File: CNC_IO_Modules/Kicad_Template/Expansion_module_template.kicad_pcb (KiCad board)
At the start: 2 copper layers, 32 x 42 mm, 2 parts

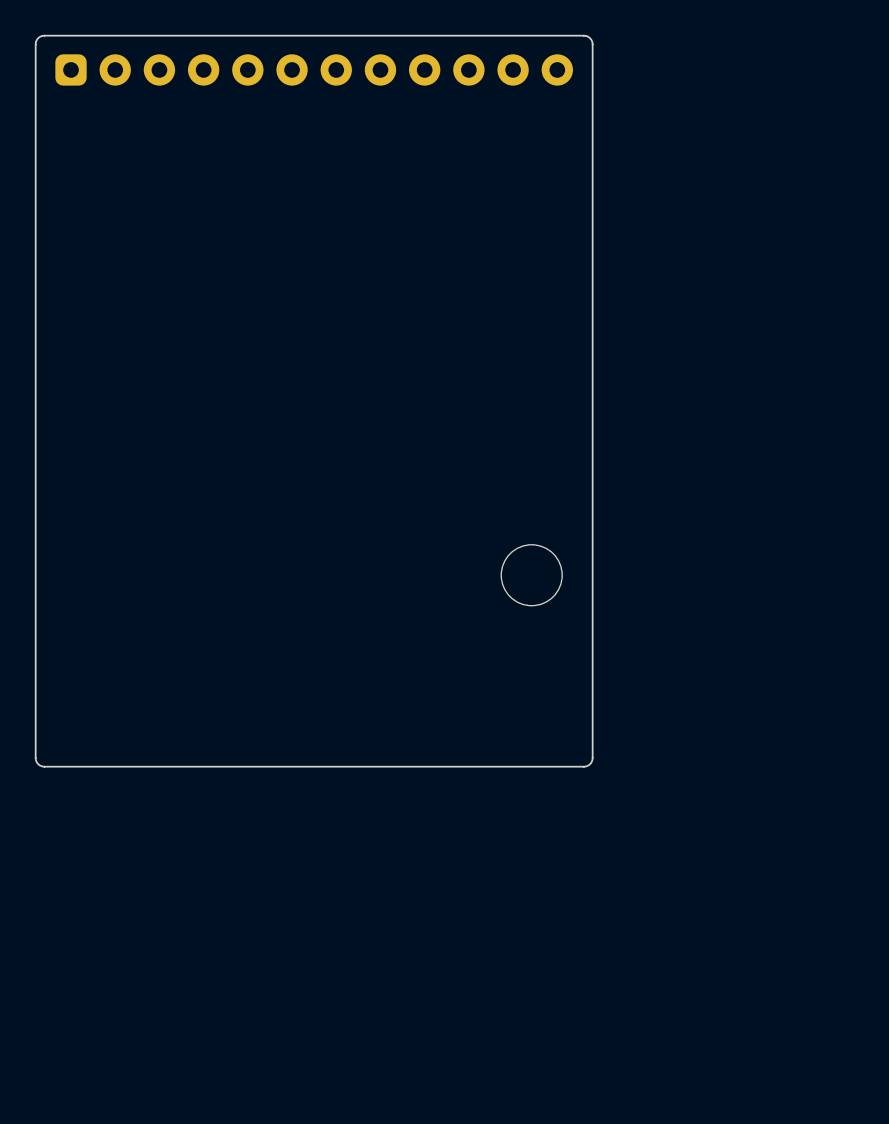
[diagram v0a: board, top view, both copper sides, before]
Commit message: Add Kicad versions
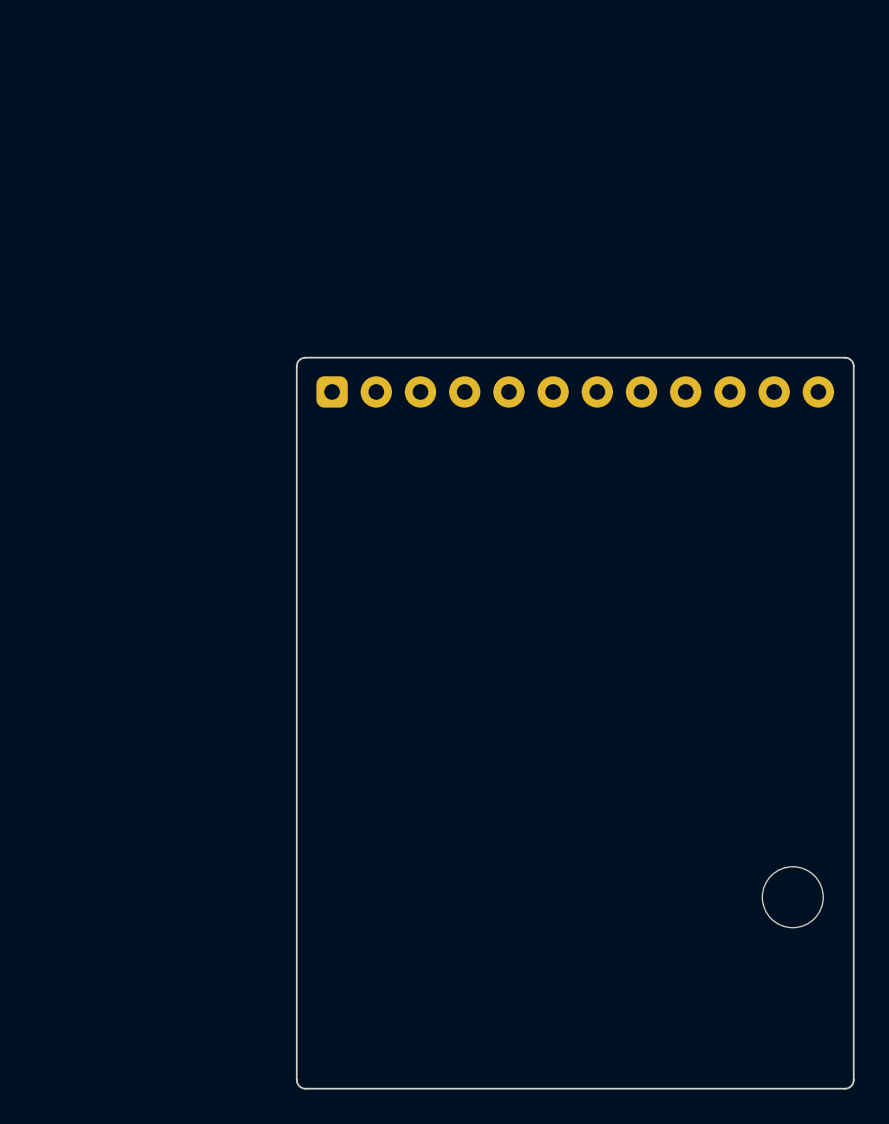
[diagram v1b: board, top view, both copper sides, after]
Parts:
- moved REF** 23.8 mm to (143.5, 107.5)
- moved REF** 23.8 mm to (117.0, 78.5)
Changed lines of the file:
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@@
   (net 0 "")
   (footprint "MountingHole:MountingHole_3.5mm" (layer "F.Cu")
-    (at 128.5 89)
+    (at 143.5 107.5)
     (descr "Mounting Hole 3.5mm, no annular")
     (tags "mounting hole 3.5mm no annular")
@@
   )
   (footprint "Connector_PinHeader_2.54mm:PinHeader_1x12_P2.54mm_Vertical" (layer "F.Cu")
-    (at 102.02998 59.97001 90)
+    (at 117.02998 78.47001 90)
     (descr "Through hole straight pin header, 1x12, 2.54mm pitch, single row")
     (tags "Through hole pin header THT 1x12 2.54mm single row")
@@
     )
   )
-  (gr_circle (center 128.49999 88.99999) (end 130.24998 88.99999) (layer "B.Mask") (width 0) (fill solid))
-  (gr_circle (center 128.49999 88.99999) (end 130.24998 88.99999) (layer "F.Mask") (width 0) (fill solid))
-  (gr_arc (start 100.5 100) (mid 100.146447 99.853553) (end 100 99.5) (layer "Edge.Cuts") (width 0.1))
-  (gr_arc (start 132 99.5) (mid 131.853553 99.853553) (end 131.5 100) (layer "Edge.Cuts") (width 0.1))
-  (gr_line (start 132 58.5) (end 132 99.5) (layer "Edge.Cuts") (width 0.1))
-  (gr_line (start 100.5 58) (end 131.5 58) (layer "Edge.Cuts") (width 0.1))
-  (gr_line (start 131.5 100) (end 100.5 100) (layer "Edge.Cuts") (width 0.1))
-  (gr_arc (start 100 58.5) (mid 100.146447 58.146447) (end 100.5 58) (layer "Edge.Cuts") (width 0.1))
-  (gr_arc (start 131.5 58) (mid 131.853553 58.146447) (end 132 58.5) (layer "Edge.Cuts") (width 0.1))
-  (gr_line (start 100 99.5) (end 100 58.5) (layer "Edge.Cuts") (width 0.1))
-  (gr_text "5" (at 119.729 56.391272) (layer "Dwgs.User")
+  (gr_circle (center 143.49999 107.49999) (end 145.24998 107.49999) (layer "B.Mask") (width 0) (fill solid))
+  (gr_circle (center 143.49999 107.49999) (end 145.24998 107.49999) (layer "F.Mask") (width 0) (fill solid))
+  (gr_arc (start 115.5 118.5) (mid 115.146447 118.353553) (end 115 118) (layer "Edge.Cuts") (width 0.1))
+  (gr_arc (start 147 118) (mid 146.853553 118.353553) (end 146.5 118.5) (layer "Edge.Cuts") (width 0.1))
+  (gr_line (start 147 77) (end 147 118) (layer "Edge.Cuts") (width 0.1))
+  (gr_line (start 115.5 76.5) (end 146.5 76.5) (layer "Edge.Cuts") (width 0.1))
+  (gr_line (start 146.5 118.5) (end 115.5 118.5) (layer "Edge.Cuts") (width 0.1))
+  (gr_arc (start 115 77) (mid 115.146447 76.646447) (end 115.5 76.5) (layer "Edge.Cuts") (width 0.1))
+  (gr_arc (start 146.5 76.5) (mid 146.853553 76.646447) (end 147 77) (layer "Edge.Cuts") (width 0.1))
+  (gr_line (start 115 118) (end 115 77) (layer "Edge.Cuts") (width 0.1))
+  (gr_text "5" (at 134.729 74.891272) (layer "Dwgs.User")
     (effects (font (size 1 1) (thickness 0.15)))
   )
-  (gr_text "3" (at 114.522 56.391272) (layer "Dwgs.User")
+  (gr_text "3" (at 129.522 74.891272) (layer "Dwgs.User")
     (effects (font (size 1 1) (thickness 0.15)))
   )
-  (gr_text "VMOT" (at 104.616 55.32901 90) (layer "Dwgs.User")
+  (gr_text "VMOT" (at 119.616 73.82901 90) (layer "Dwgs.User")
     (effects (font (size 1 1) (thickness 0.15)))
   )
-  (gr_text "GND" (at 130.016 55.709963 90) (layer "Dwgs.User")
+  (gr_text "GND" (at 145.016 74.209963 90) (layer "Dwgs.User")
     (effects (font (size 1 1) (thickness 0.15)))
   )
-  (gr_text "7" (at 124.809 56.391272) (layer "Dwgs.User")
+  (gr_text "7" (at 139.809 74.891272) (layer "Dwgs.User")
     (effects (font (size 1 1) (thickness 0.15)))
   )
-  (gr_text "8" (at 127.476 56.391272) (layer "Dwgs.User")
+  (gr_text "8" (at 142.476 74.891272) (layer "Dwgs.User")
     (effects (font (size 1 1) (thickness 0.15)))
   )
-  (gr_text "5V" (at 107.156 56.32901 90) (layer "Dwgs.User")
+  (gr_text "5V" (at 122.156 74.82901 90) (layer "Dwgs.User")
     (effects (font (size 1 1) (thickness 0.15)))
   )
-  (gr_text "6" (at 122.396 56.391272) (layer "Dwgs.User")
+  (gr_text "6" (at 137.396 74.891272) (layer "Dwgs.User")
     (effects (font (size 1 1) (thickness 0.15)))
   )
-  (gr_text "2" (at 112.109 56.391272) (layer "Dwgs.User")
+  (gr_text "2" (at 127.109 74.891272) (layer "Dwgs.User")
     (effects (font (size 1 1) (thickness 0.15)))
   )
-  (gr_text "1" (at 109.569 56.391272) (layer "Dwgs.User")
+  (gr_text "1" (at 124.569 74.891272) (layer "Dwgs.User")
     (effects (font (size 1 1) (thickness 0.15)))
   )
-  (gr_text "4" (at 117.189 56.391272) (layer "Dwgs.User")
+  (gr_text "4" (at 132.189 74.891272) (layer "Dwgs.User")
     (effects (font (size 1 1) (thickness 0.15)))
   )
-  (gr_text "GND" (at 102.076 55.709963 90) (layer "Dwgs.User")
+  (gr_text "GND" (at 117.076 74.209963 90) (layer "Dwgs.User")
     (effects (font (size 1 1) (thickness 0.15)))
   )
+  (dimension (type aligned) (layer "Dwgs.User")
+    (pts (xy 115 118) (xy 147 118))
+    (height 5.12)
+    (gr_text "32,0000 mm" (at 131 121.97) (layer "Dwgs.User")
+      (effects (font (size 1 1) (thickness 0.15)))
+    )
+    (format (units 3) (units_format 1) (precision 4))
+    (style (thickness 0.1) (arrow_length 1.27) (text_position_mode 0) (extension_height 0.58642) (extension_offset 0.5) keep_text_aligned)
+  )
+  (dimension (type aligned) (layer "Dwgs.User")
+    (pts (xy 146.5 118.5) (xy 146.5 76.5))
+    (height 6.05)
+    (gr_text "42,0000 mm" (at 151.4 97.5 90) (layer "Dwgs.User")
+      (effects (font (size 1 1) (thickness 0.15)))
+    )
+    (format (units 3) (units_format 1) (precision 4))
+    (style (thickness 0.1) (arrow_length 1.27) (text_position_mode 0) (extension_height 0.58642) (extension_offset 0.5) keep_text_aligned)
+  )
+  (dimension (type aligned) (layer "Dwgs.User")
+    (pts (xy 147 118.5) (xy 147 107.5))
+    (height 11)
+    (gr_text "11,0000 mm" (at 156.85 113 90) (layer "Dwgs.User")
+      (effects (font (size 1 1) (thickness 0.15)))
+    )
+    (format (units 3) (units_format 1) (precision 4))
+    (style (thickness 0.1) (arrow_length 1.27) (text_position_mode 0) (extension_height 0.58642) (extension_offset 0.5) keep_text_aligned)
+  )
 )
